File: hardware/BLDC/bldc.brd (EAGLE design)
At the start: 51 x 40 mm, 84 parts, among them J1 PWR_2_XT30PW-M, J2 LINEAR_3_JST_PH_RA, J3 LINEAR_8_JST_PH_RA, U1 MA702, U10 MCP2542FD, U11 LDFM33PUR, U2 DRV8323RS, U3 TPN7R006PL, U4 TPN7R006PL, U5 TPN7R006PL, U6 TPN7R006PL, U7 TPN7R006PL, U8 TPN7R006PL, U9 STM32G4_UFQFPN48_T1, X1 CRYSTAL_NX2016SA-24MHZ-EXS00A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

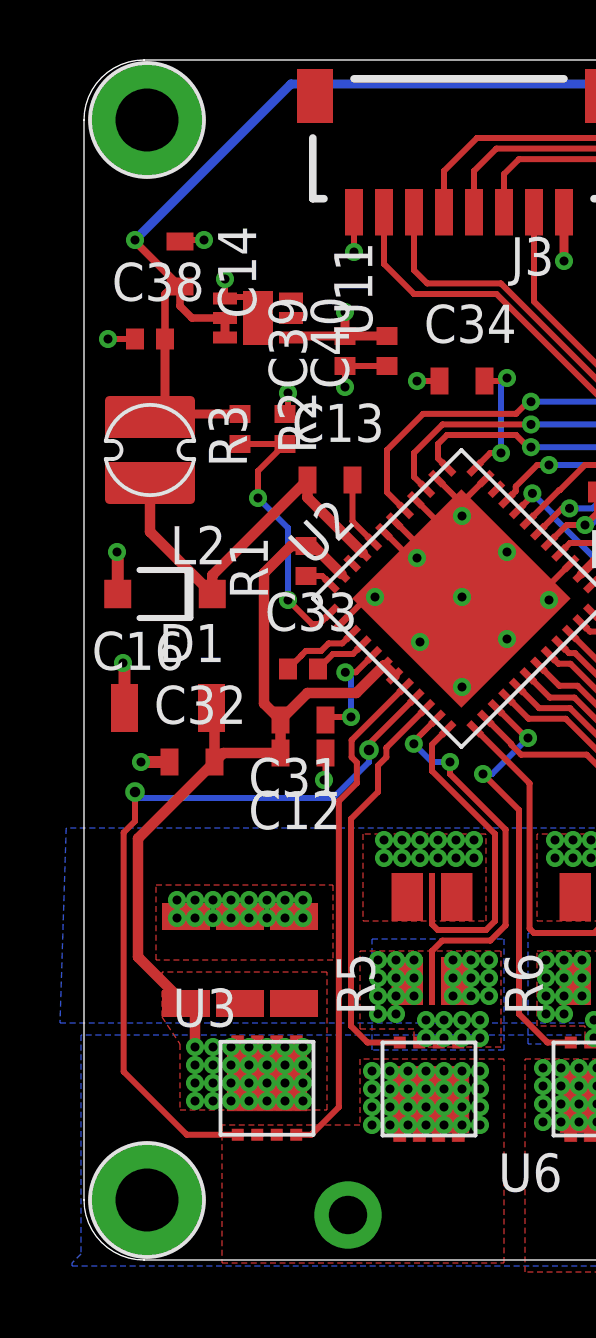
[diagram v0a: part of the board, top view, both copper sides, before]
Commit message: Prior to BOM consolidation
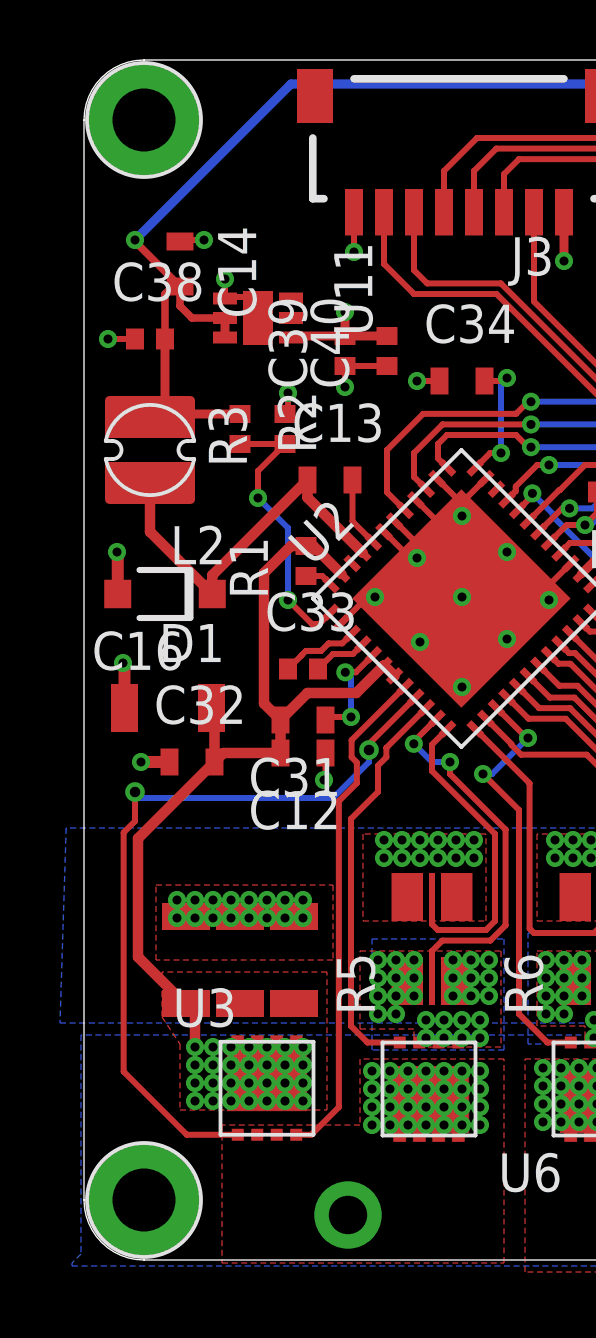
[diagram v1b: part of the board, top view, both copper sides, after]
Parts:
- moved H1 0.10 mm to (2.00, 2.00)
- moved H2 0.10 mm to (2.00, 38.0)
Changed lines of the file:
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@@
 <layer number="1" name="Top" color="4" fill="1" visible="yes" active="yes"/>
 <layer number="2" name="Route2" color="16" fill="1" visible="yes" active="yes"/>
-<layer number="15" name="Route15" color="23" fill="1" visible="no" active="yes"/>
+<layer number="15" name="Route15" color="23" fill="1" visible="yes" active="yes"/>
 <layer number="16" name="Bottom" color="1" fill="1" visible="yes" active="yes"/>
 <layer number="17" name="Pads" color="2" fill="1" visible="yes" active="yes"/>
@@
 </layers>
 <board>
-<fusionsync huburn="a.YnVzaW5lc3M6Z21haWwyMjE5MTc" projecturn="a.YnVzaW5lc3M6Z21haWwyMjE5MTcjMjAxOTA2MjkyMDE0MTU5NzY" f3durn="urn:adsk.wipprod:dm.lineage:e4urj2y-ReajaBtUk_DaUw" pcbguid="" lastpulledtime="" lastsyncedchangeguid="" latestrevisionid="c8898aa8-4816-4024-a727-549153469479" lastsyncedrevisionid="c8898aa8-4816-4024-a727-549153469479" lastboardhashguid="96ba5604-6864-0f3b-cda7-083015d9c990" lastpushedtime="2020-05-19T04:17:52Z" linktopcb3d="%12"/>
+<fusionsync huburn="a.YnVzaW5lc3M6Z21haWwyMjE5MTc" projecturn="a.YnVzaW5lc3M6Z21haWwyMjE5MTcjMjAxOTA2MjkyMDE0MTU5NzY" f3durn="urn:adsk.wipprod:dm.lineage:e4urj2y-ReajaBtUk_DaUw" pcbguid="" lastpulledtime="" lastsyncedchangeguid="" latestrevisionid="0cfa6979-0abf-47e5-904f-7e41c382e9f9" lastsyncedrevisionid="0cfa6979-0abf-47e5-904f-7e41c382e9f9" lastboardhashguid="129d7aed-9189-2586-7fe0-9e496c46e9fb" lastpushedtime="2020-05-19T04:37:09Z" linktopcb3d="%12"/>
 <plain>
 <wire x1="39.0836" y1="39.681" x2="38" y2="40" width="0" layer="20" curve="32.8049"/>
@@
 <attribute name="VALUE" x="36.65" y="8.95" size="1.27" layer="27" rot="R180"/>
 </element>
-<element name="H1" library="_T_conn" library_urn="urn:adsk.eagle:library:19570503" package="M2" package3d_urn="urn:adsk.eagle:package:20293119/4" value="PCB_MOUNT_HOLE_M2" x="2.1" y="2" smashed="yes"/>
-<element name="H2" library="_T_conn" library_urn="urn:adsk.eagle:library:19570503" package="M2" package3d_urn="urn:adsk.eagle:package:20293119/4" value="PCB_MOUNT_HOLE_M2" x="2.1" y="38" smashed="yes"/>
+<element name="H1" library="_T_conn" library_urn="urn:adsk.eagle:library:19570503" package="M2" package3d_urn="urn:adsk.eagle:package:20293119/4" value="PCB_MOUNT_HOLE_M2" x="2" y="2" smashed="yes"/>
+<element name="H2" library="_T_conn" library_urn="urn:adsk.eagle:library:19570503" package="M2" package3d_urn="urn:adsk.eagle:package:20293119/4" value="PCB_MOUNT_HOLE_M2" x="2" y="38" smashed="yes"/>
 <element name="H3" library="_T_conn" library_urn="urn:adsk.eagle:library:19570503" package="M2" package3d_urn="urn:adsk.eagle:package:20293119/4" value="PCB_MOUNT_HOLE_M2" x="38" y="2" smashed="yes"/>
 <element name="H4" library="_T_conn" library_urn="urn:adsk.eagle:library:19570503" package="M2" package3d_urn="urn:adsk.eagle:package:20293119/4" value="PCB_MOUNT_HOLE_M2" x="38" y="38" smashed="yes"/>
